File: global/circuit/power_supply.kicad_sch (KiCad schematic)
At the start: 20 parts, among them U1 LMR62014XMF-NOPB, U5 TLV767

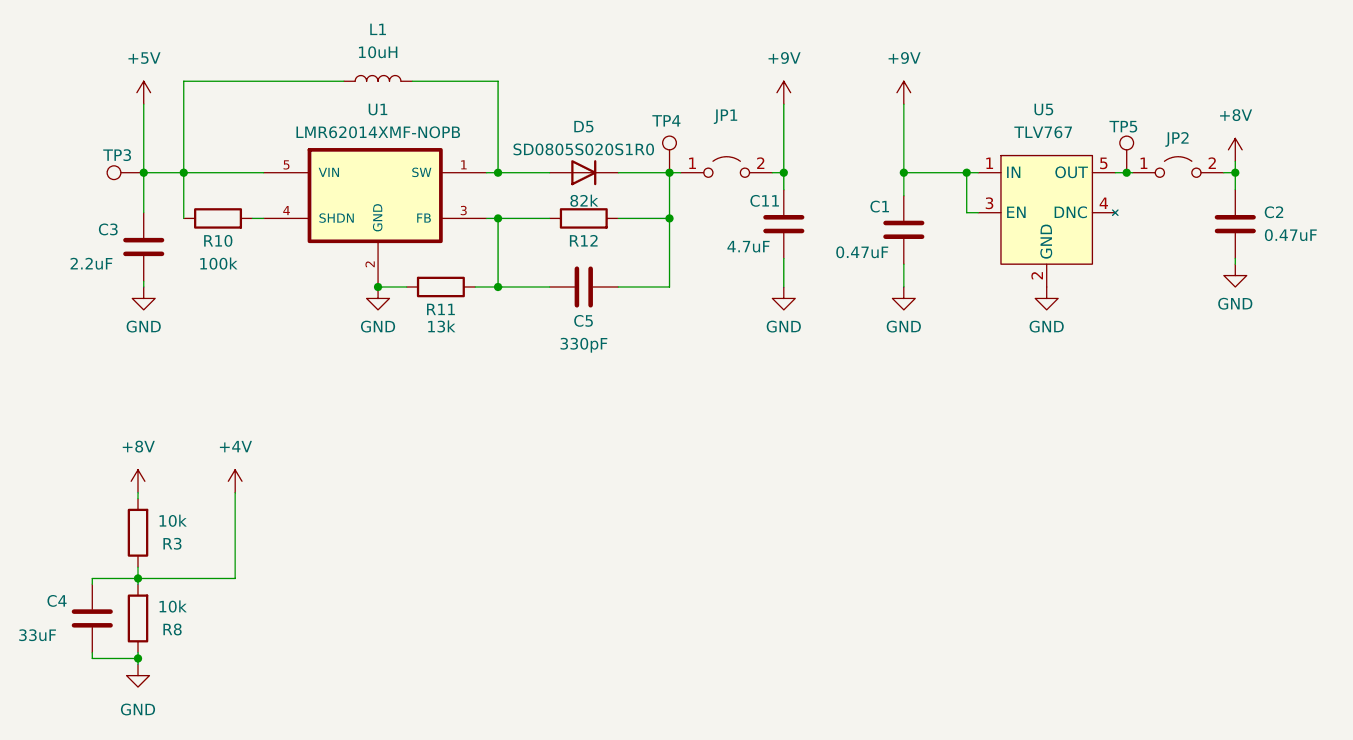
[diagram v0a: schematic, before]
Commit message: rework global circuits
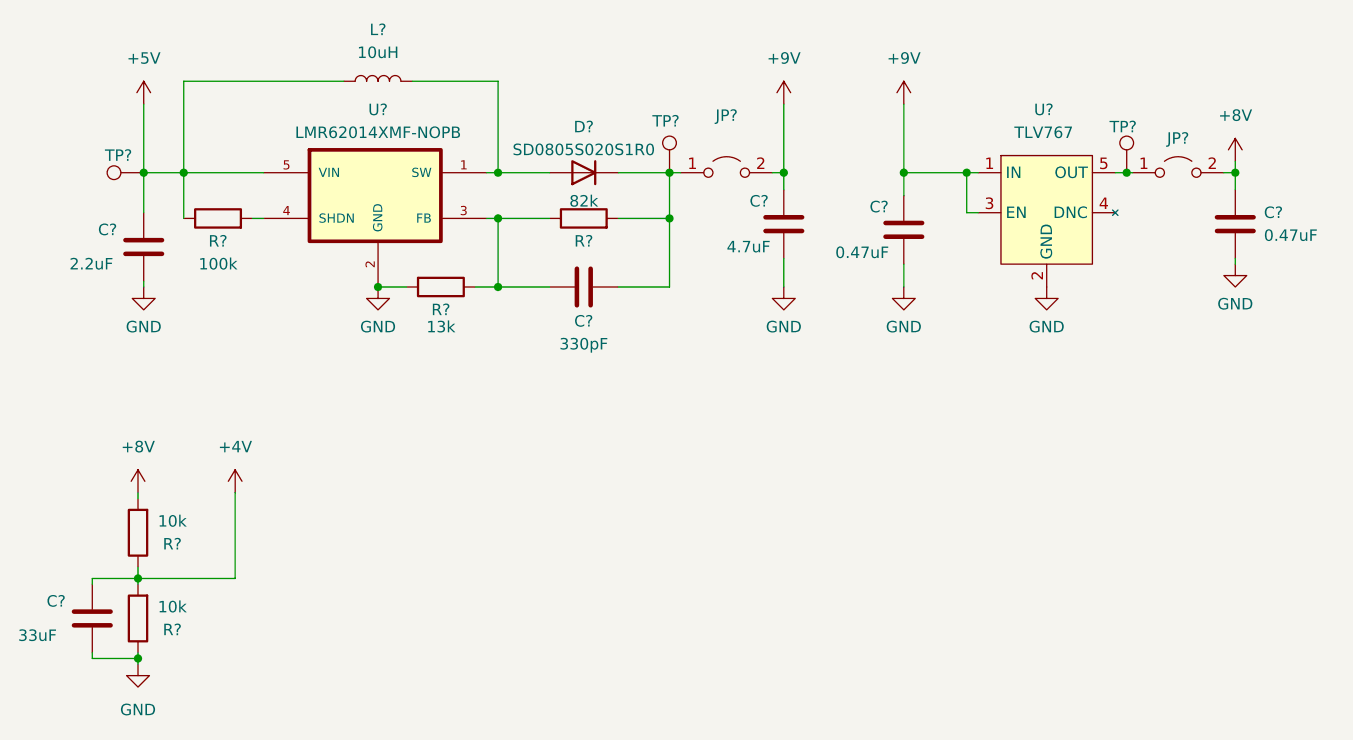
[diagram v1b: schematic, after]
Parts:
- L?: renamed from L1; footprint Inductor_SMD:L_Abracon_ASPI-3012S -> Inductor_SMD:L_0805_2012Metric_Pad1.15x1.40mm_HandSolder
- renumbered C2 to C?, C5 to C?, C4 to C?, C3 to C?, C11 to C?, C1 to C?, D5 to D?, JP1 to JP?, JP2 to JP?, R3 to R?, R10 to R?, R11 to R?, R12 to R?, R8 to R?, TP3 to TP?, TP5 to TP?, TP4 to TP?, U5 to U?, U1 to U?
